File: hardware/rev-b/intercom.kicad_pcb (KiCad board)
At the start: 2 copper layers, 66.5 x 64.5 mm, 67 parts, among them J1 Conn_02x02_Odd_Even, J2 USB_C_Receptacle_USB2.0_16P, J3 UART, J4 PTT, SW2 POWER, SW3 EN, SW4 BOOT, U1 MAX98357A, U2 TPS61088, U3 ESP32-S3-WROOM-1, U4 AP2112K-3.3, U5 MCP73831-2-OT, U6 USBLC6-2SC6

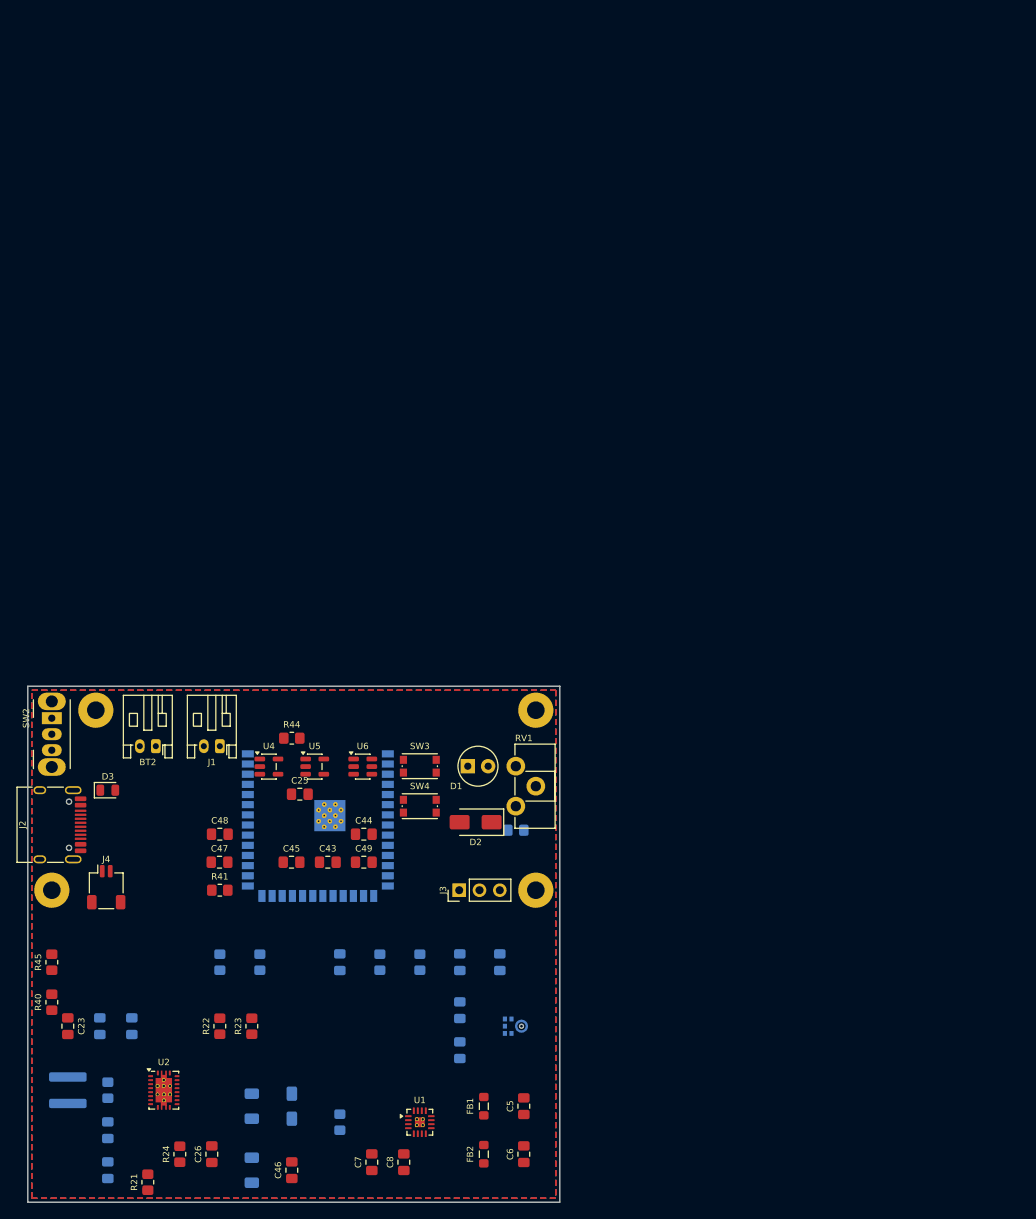
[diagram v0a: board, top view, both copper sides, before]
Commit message: update rev-b
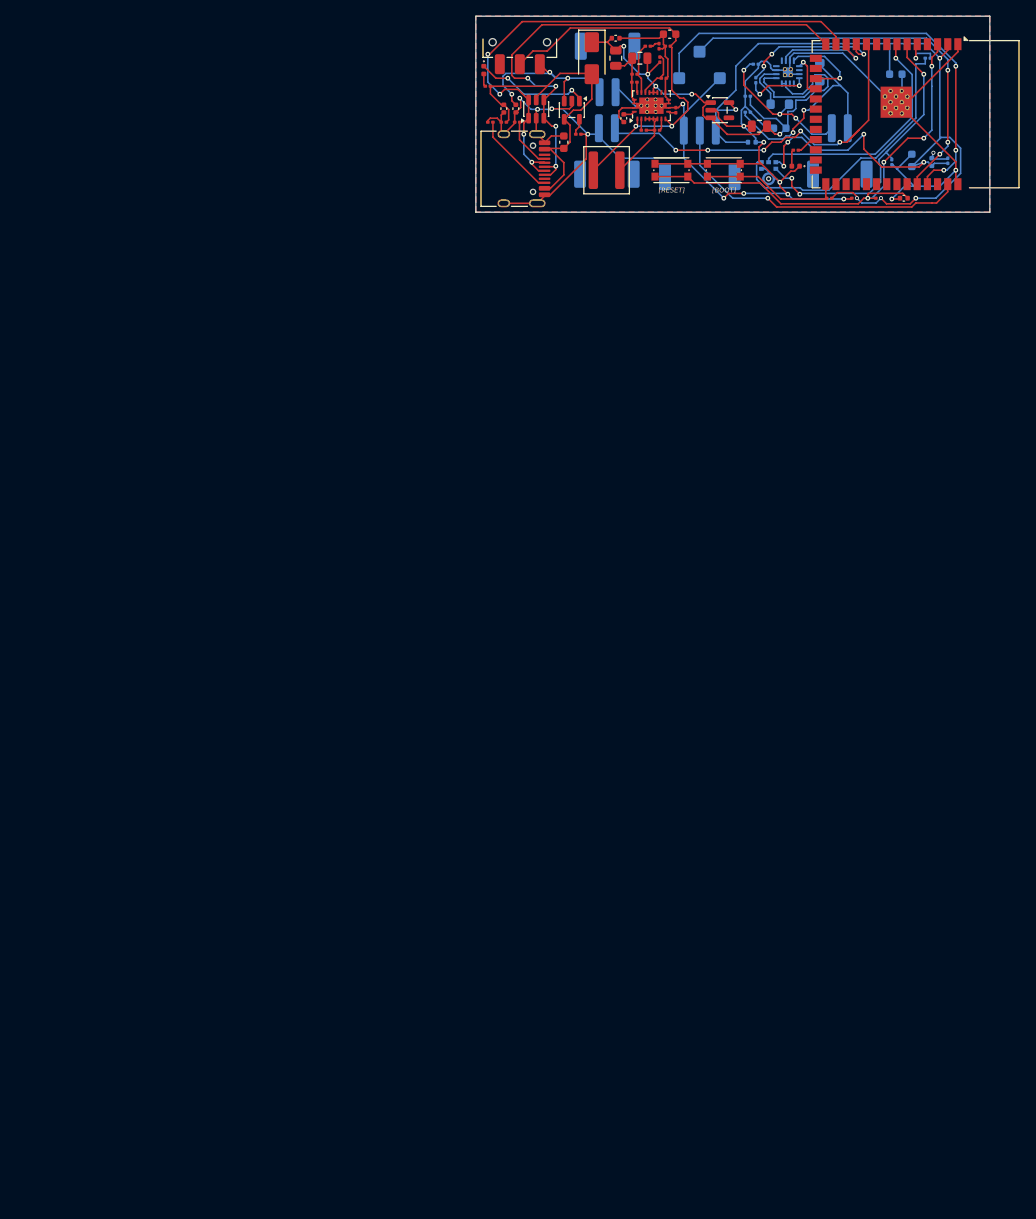
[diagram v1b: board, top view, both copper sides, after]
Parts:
- removed H1, H2, H3, H4: MountingHole_Pad, MountingHole_2.2mm_M2_Pad
- removed RV1: A50K, Potentiometer_THT:Potentiometer_Piher_PT-10-H01_Horizontal
- added J5: VOLUME BREAKOUT, Connector_JST:JST_PH_S3B-PH-SM4-TB_1x03-1MP_P2.00mm_Horizontal, B.Cu at (215.0, 48.9)
- BT2, J1: footprint JST_PH_S2B-PH-K_1x02_P2.00mm_Horizontal -> Connector_JST:JST_PH_S2B-PH-SM4-TB_1x02-1MP_P2.00mm_Horizontal; moved to B.Cu
- C2, C23, C43, C45, C46: footprint Capacitor_SMD:C_0805_2012Metric_Pad1.18x1.45mm_HandSolder -> Capacitor_SMD:C_0402_1005Metric
- C22, C24, C31, C41: footprint Capacitor_SMD:C_0805_2012Metric_Pad1.18x1.45mm_HandSolder -> Capacitor_SMD:C_0201_0603Metric; moved to F.Cu
- C25, C26, C3, C48: footprint Capacitor_SMD:C_0805_2012Metric_Pad1.18x1.45mm_HandSolder -> Capacitor_SMD:C_0201_0603Metric
- C27, C28, C29: footprint Capacitor_SMD:C_1206_3216Metric_Pad1.33x1.80mm_HandSolder -> Capacitor_SMD:C_0805_2012Metric; moved to F.Cu
- C30: footprint Capacitor_SMD:C_0805_2012Metric_Pad1.18x1.45mm_HandSolder -> Capacitor_SMD:C_0603_1608Metric; moved to F.Cu
- C40, C47: footprint Capacitor_SMD:C_0805_2012Metric_Pad1.18x1.45mm_HandSolder -> Capacitor_SMD:C_0603_1608Metric
- C42: footprint Capacitor_SMD:C_0805_2012Metric_Pad1.18x1.45mm_HandSolder -> Capacitor_SMD:C_0402_1005Metric; moved to F.Cu
- C44: footprint Capacitor_SMD:C_0805_2012Metric_Pad1.18x1.45mm_HandSolder -> Capacitor_SMD:C_0402_1005Metric; moved to B.Cu
- C49, C8: footprint Capacitor_SMD:C_0805_2012Metric_Pad1.18x1.45mm_HandSolder -> Capacitor_SMD:C_0603_1608Metric; moved to B.Cu
- C5, C6, C7: footprint Capacitor_SMD:C_0805_2012Metric_Pad1.18x1.45mm_HandSolder -> Capacitor_SMD:C_0201_0603Metric; moved to B.Cu
- D1: footprint LED_D5.0mm -> LED_SMD:LED_0402_1005Metric
- D3: footprint LED_SMD:LED_0805_2012Metric -> LED_SMD:LED_0402_1005Metric
- FB1, FB2: moved to B.Cu
- J3: value UART -> UART TEST PADS; footprint Connector_PinHeader_2.54mm:PinHeader_1x03_P2.54mm_Vertical -> Intercom:UART_TestPads_3Pin; moved to B.Cu
- J4: value PTT -> PTT BREAKOUT; footprint Connector_JST:JST_SH_SM02B-SRSS-TB_1x02-1MP_P1.00mm_Horizontal -> Connector_JST:JST_PH_S2B-PH-SM4-TB_1x02-1MP_P2.00mm_Horizontal; moved to B.Cu
- L2: value 1.2uH -> XAL5030-122MEC; moved to F.Cu
- R1, R20, R42, R43: footprint Resistor_SMD:R_0805_2012Metric_Pad1.20x1.40mm_HandSolder -> Resistor_SMD:R_0201_0603Metric; moved to F.Cu
- R2, R21, R22, R23, R24, R3, R40, R41, R44, R45: footprint Resistor_SMD:R_0805_2012Metric_Pad1.20x1.40mm_HandSolder -> Resistor_SMD:R_0201_0603Metric
- R4: value 1M -> 0; footprint Resistor_SMD:R_0805_2012Metric_Pad1.20x1.40mm_HandSolder -> Resistor_SMD:R_0201_0603Metric
- SW2: value POWER -> JS102011SAQN; footprint Button_Switch_THT:SW_Slide_SPDT_Angled_CK_OS102011MA1Q -> Button_Switch_SMD:SW_SPDT_CK_JS102011SAQN
- SW3: value EN -> KMR231GLFS
- SW4: value BOOT -> KMR231GLFS
- U1: value MAX98357A -> MAX98357AETE+T; moved to B.Cu
- U2: value TPS61088 -> TPS61088RHLR
- U3: value ESP32-S3-WROOM-1 -> ESP32-S3-WROOM-1-N8R8; moved to F.Cu
- U4: value AP2112K-3.3 -> AP2112K-3.3TRG1
- U5: value MCP73831-2-OT -> MCP73831T-2ACI/OT
- moved R21 150.4 mm to (206.8, 40.0), turned to 180 degrees
- moved R24 150.3 mm to (208.5, 35.5), turned to 0 degrees
- moved C24 150.3 mm to (212.0, 43.5)
- moved C27 145.1 mm to (222.4, 45.5), turned to 180 degrees
- moved C26 145.0 mm to (206.8, 39.0), turned to 180 degrees
- moved C22 142.6 mm to (209.7, 46.0), turned to 180 degrees
- moved C31 141.6 mm to (211.0, 35.5), turned to 180 degrees
- moved C7 141.3 mm to (221.0, 41.8), turned to 0 degrees
- moved C30 141.1 mm to (211.2, 34.0), turned to 180 degrees
- moved R4 140.2 mm to (222.0, 39.8)
- moved C28 139.7 mm to (207.5, 37.0), turned to 180 degrees
- moved C6 139.3 mm to (222.0, 37.8), turned to 180 degrees
- moved U1 139.1 mm to (226.0, 38.8), turned to 180 degrees
- moved C8 137.5 mm to (225.0, 45.8), turned to 0 degrees
- moved R20 137.4 mm to (208.0, 46.0), turned to 180 degrees
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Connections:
- C2 pad 1: Net-(MK1-VDD) -> +3.3V
- C2 pad 2: +3.3V -> GND
- C3 pad 1: Net-(MK1-VDD) -> +3.3V
- C3 pad 2: +3.3V -> GND
- MK1 pad 1: MIC_WS -> Net-(MK1-WS)
- MK1 pad 5: Net-(MK1-VDD) -> +3.3V
- R3 pad 2: MIC_WS -> Net-(MK1-WS)
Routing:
- net GND: track 0.00 -> 256.4 mm, vias 0 -> 15
- net +3.3V: track 0.00 -> 122.8 mm, vias 0 -> 9
- net USB_DN: track 0.00 -> 69.2 mm, vias 0 -> 4
- net +5V: track 0.00 -> 66.2 mm, vias 0 -> 5
- net USB_DP: track 0.00 -> 65.9 mm, vias 0 -> 4
- net ESP_EN: track 0.00 -> 59.4 mm, vias 0 -> 4
- net U0TXD: track 0.00 -> 57.8 mm, vias 0 -> 3
- net U0RXD: track 0.00 -> 50.0 mm, vias 0 -> 3
- net /Power/VBAT: track 0.00 -> 49.9 mm, vias 0 -> 2
- net PTT: track 0.00 -> 47.3 mm, vias 0 -> 5
- net VBUS: track 0.00 -> 43.7 mm
- net VOLUME: track 0.00 -> 39.0 mm, vias 0 -> 1
- net MIC_BCLK: track 0.00 -> 37.7 mm, vias 0 -> 3
- net Net-(MK1-WS): track 0.00 -> 35.6 mm
- net MIC_SD: track 0.00 -> 30.6 mm, vias 0 -> 1
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- removed copper zone on B.Cu, net +5V
- removed copper zone on F.Cu, net +5V
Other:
- board size 66.5 x 64.5 mm -> 64.2 x 24.5 mm
- board text added: "Arbiter Intercom REV-B, Designed By Tyler Reckart, August 2026"
- board text added: "BTY"
- board text added: "MIC"
- board text added: "PTT"
- board text added: "SPKR"
- board text added: "VOL"
- board text added: "[BOOT]"
- board text added: "[RESET]"
